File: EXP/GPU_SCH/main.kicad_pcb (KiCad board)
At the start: 2 copper layers, 137.2 x 76.4 mm, 67 parts, among them J1 Conn_02x10_Counter_Clockwise, J2 Conn_01x03, J6 DB15_Female_HighDensity, Q1 FDV301N, Q2 FDV301N, Q3 FDV301N, U1 74HC4040, U10 74LS157, U11 74HC688, U12 74HC688, U13 74LS157, U14 74LS157, U15 74HC688, U16 74HC688, U17 74LS157, U18 74HC373, U19 74HC373, U2 74HC74, U20 74HC373, U21 74LS20, U22 74LS151, U23 74HC373, U24 74HC74, U25 74HC00, U3 74HC14, U4 74HC4040, U5 IS6xC1024AL-xxT, U6 74HC238, U7 74HC688, U8 74HC688, U9 74HC373, Y2 CXO_DIP8

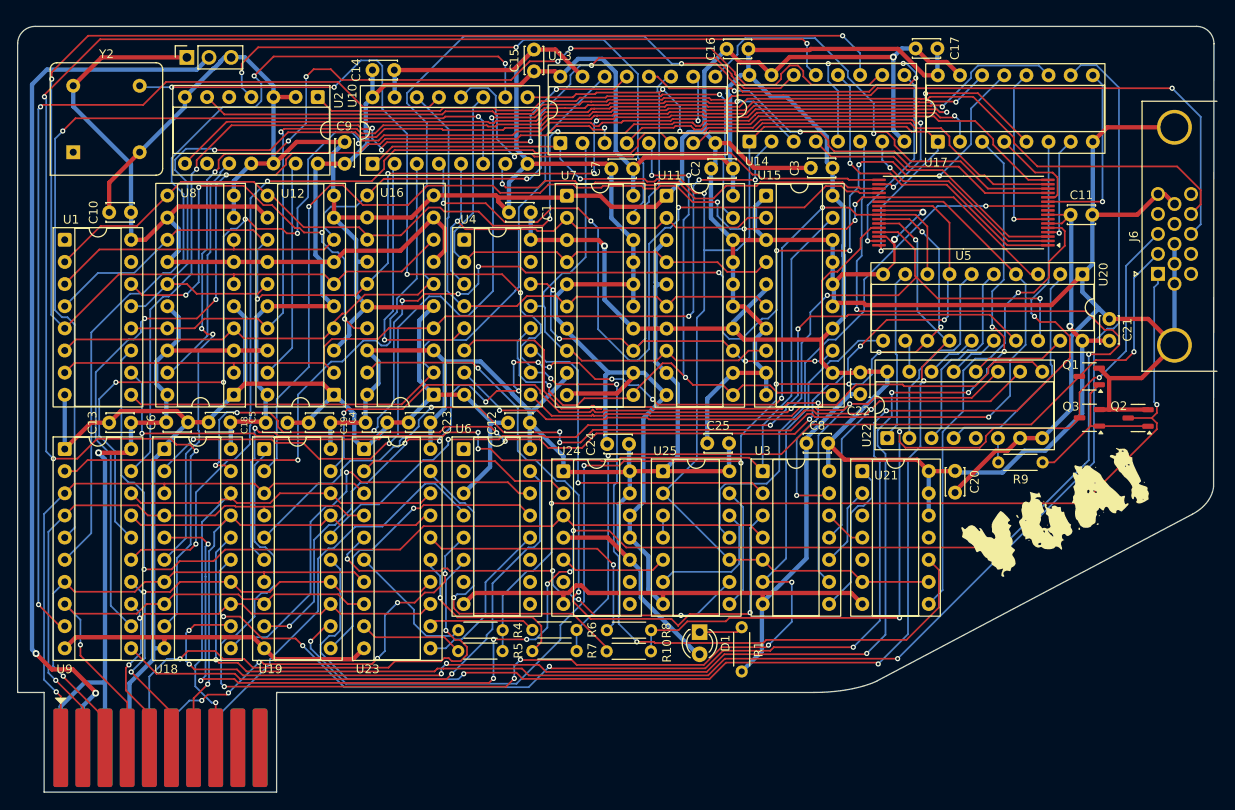
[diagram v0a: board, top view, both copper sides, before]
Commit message: Add files via upload
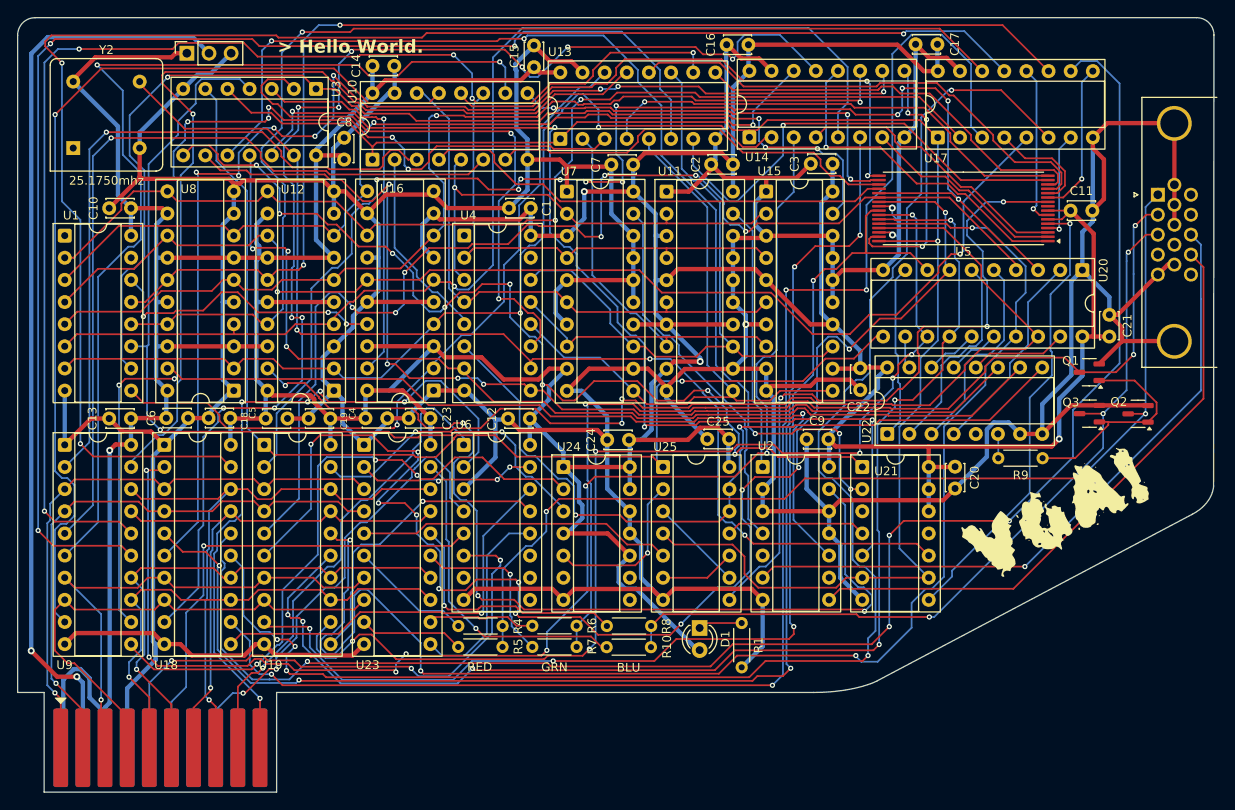
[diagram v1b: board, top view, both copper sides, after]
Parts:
- J6: footprint Connector_Dsub:DSUB-15-HD_Pins_Horizontal_P2.29x1.90mm_EdgePinOffset3.03mm_Housed_MountingHolesOffset4.94mm -> Connector_Dsub:DSUB-15-HD_Socket_Horizontal_P2.29x1.90mm_EdgePinOffset3.03mm_Housed_MountingHolesOffset4.94mm
- Y2: value CXO_DIP8 -> 25.1750mhz
- moved U3 67.4 mm to (88.0, 91.7), turned to -90 degrees
- moved U2 66.4 mm to (139.3, 135.1), turned to 0 degrees
- moved C8 64.4 mm to (91.2, 99.8), turned to 90 degrees
- moved C9 63.9 mm to (146.8, 131.9), turned to 180 degrees
- moved J6 9.08 mm to (184.6, 103.9)
- moved C10 0.48 mm to (64.3, 105.4)
- moved C12 0.48 mm to (110.0, 129.5)
- moved C15 0.48 mm to (113.0, 89.2)
- moved C16 0.48 mm to (137.6, 86.7)
- moved C17 0.48 mm to (159.3, 86.6)
- moved C18 0.48 mm to (75.7, 129.5)
- moved C23 0.48 mm to (98.7, 129.5)
- moved C24 0.48 mm to (123.9, 132.0)
- moved C25 0.48 mm to (135.4, 131.9)
- moved C4 0.48 mm to (93.7, 129.5)
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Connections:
- U25 pad 1: +5V -> PRE
- U25 pad 10: ~{PRE} -> Net-(U25-Pad10)
- U25 pad 11: A16 -> Net-(U21-Pad4)
- U25 pad 12: Net-(U25-Pad12) -> /X2
- U25 pad 13: Net-(U25-Pad13) -> /X2
- U25 pad 2: ~{PRE} -> F_OUT
- U25 pad 4: Net-(U25-Pad3) -> ~{PRE}
- U25 pad 5: F_OUT -> F_EDIT
- U25 pad 6: Net-(U25-Pad12) -> Net-(U25-Pad10)
- U25 pad 8: Net-(U25-Pad13) -> A16
- U25 pad 9: F_EDIT -> Net-(U25-Pad3)
- U3 pad 12: Net-(U21-Pad4) -> ~{VCLK}
- U3 pad 13: /X2 -> VCLK
- U6 pad 1: unconnected-(U6-A0-Pad1) -> /A0
- U6 pad 2: unconnected-(U6-A1-Pad2) -> /A1
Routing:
- net ~{VCLK}: track 0.00 -> 119.3 mm, vias 0 -> 4
- net Net-(U21-Pad2): track 9.20 -> 125.1 mm, vias 0 -> 5
- net Net-(U21-Pad1): track 18.1 -> 111.0 mm, vias 0 -> 8
- net Net-(U12-P=R): track 25.3 -> 111.3 mm, vias 0 -> 4
- net /A1: track 0.00 -> 81.0 mm, vias 0 -> 5
- net Net-(U2B-~{S}): track 27.1 -> 94.2 mm, vias 0 -> 1
- net /Y3: track 176.4 -> 116.9 mm
- net /PY2: track 212.0 -> 152.6 mm, vias 11 -> 5
- net VSYNC: track 128.0 -> 69.6 mm
- net /PD6: track 109.6 -> 165.3 mm, vias 3 -> 4
- net /A0: track 0.00 -> 55.2 mm, vias 0 -> 1
- net GND: track 882.0 -> 827.6 mm
- net HSYNC: track 131.7 -> 77.5 mm
- net /PX8: track 103.8 -> 150.1 mm, vias 2 -> 3
- net /X0: track 79.7 -> 120.2 mm, vias 1 -> 4
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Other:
- board size 137.2 x 76.4 mm -> 137.2 x 77.4 mm
- board text added: "> Hello World."
- board text added: "BLU"
- board text added: "GRN"
- board text added: "RED"
